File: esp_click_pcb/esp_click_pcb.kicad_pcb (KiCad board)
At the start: 2 copper layers, 90 x 60 mm, 53 parts, among them J1 USB_C, SW1 BOOT, SW2 FLASH, SW3 BT1, SW4 BT2, SW5 BT3, SW6 BT4, U1 ESP32-C6-MINI, U2 HT7833, U4 BQ24075RGT

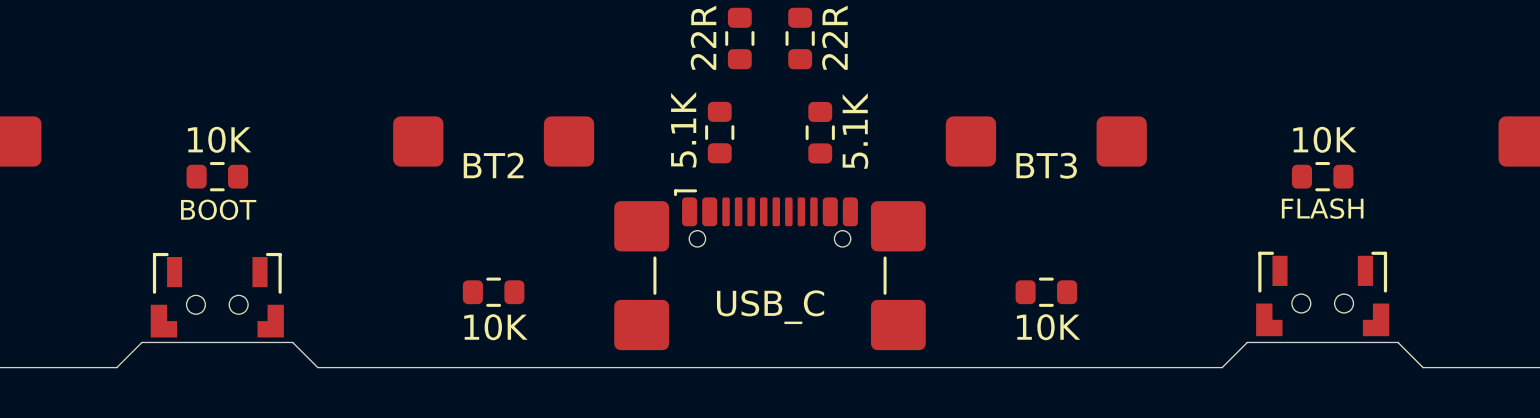
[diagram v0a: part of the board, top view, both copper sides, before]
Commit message: layout finished pcb
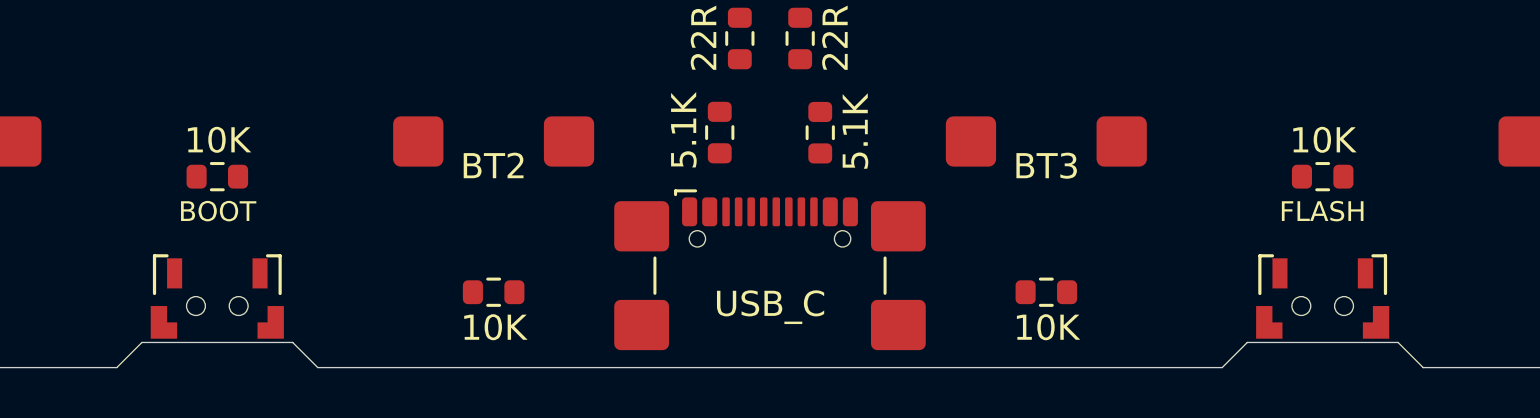
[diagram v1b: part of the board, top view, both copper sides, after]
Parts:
- moved SW2 0.10 mm to (172.0, 127.5)
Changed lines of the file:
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@@
 	(footprint "TS-A002:TST-A002_0.6MM_BOSS"
 		(layer "F.Cu")
-		(at 128 127.5 180)
+		(at 128 127.55 180)
 		(property "Reference" "SW1"
 			(at 1 3 0)
@@
 	(footprint "TS-A002:TST-A002_0.6MM_BOSS"
 		(layer "F.Cu")
-		(at 172 127.45 180)
+		(at 172 127.55 180)
 		(property "Reference" "SW2"
 			(at 1 3 0)
